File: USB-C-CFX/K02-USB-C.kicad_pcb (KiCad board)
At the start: 2 copper layers, 98.3 x 87.7 mm, 31 parts, among them SW1 SW_Push, SW10 SW_Push, SW11 SW_Push, SW12 SW_Push, SW13 SW_Push, SW14 SW_Push, SW15 SW_Push, SW16 SW_Push, SW17 SW_Push, SW18 SW_Push, SW2 SW_Push, SW3 SW_Push, SW4 SW_Push, SW5 SW_Push, SW6 SW_Push, SW7 SW_Push, SW8 SW_Push, SW9 SW_Push, U1 ProMicro-kbd

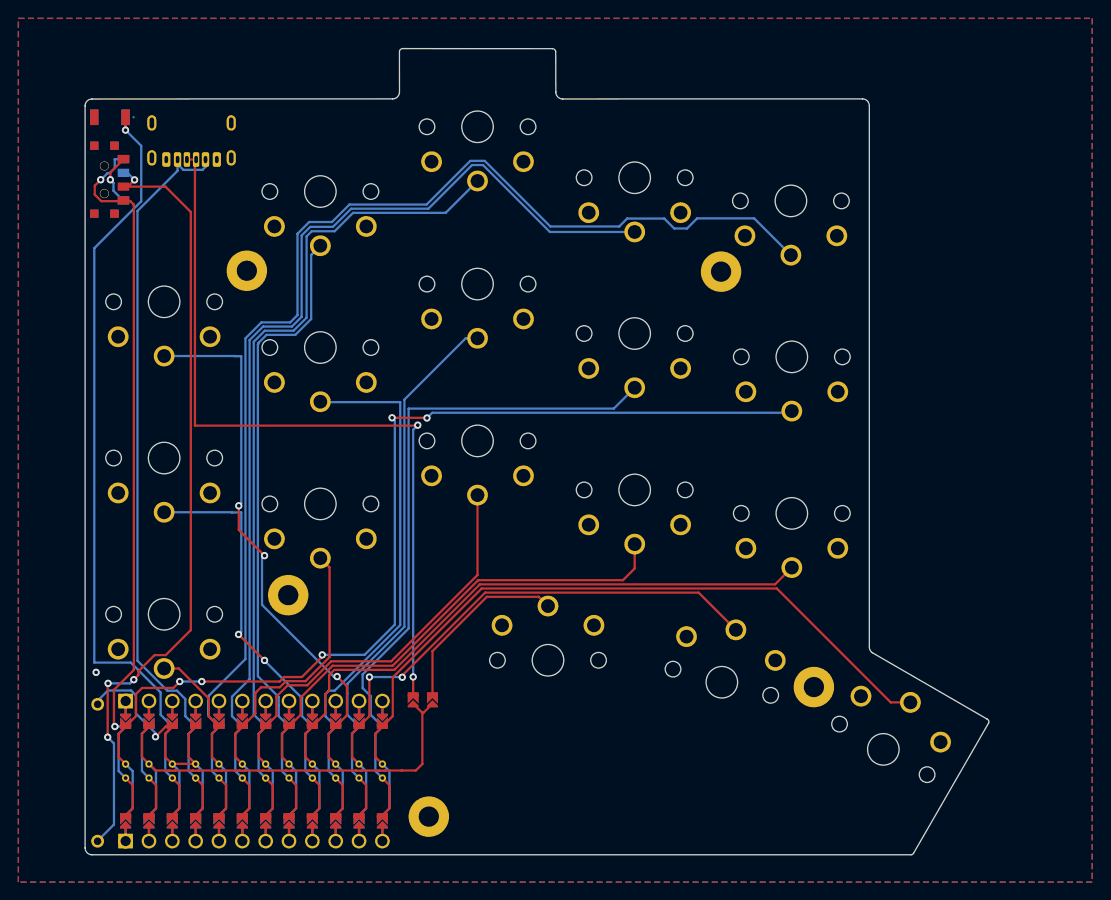
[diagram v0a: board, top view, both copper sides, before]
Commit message: upsie
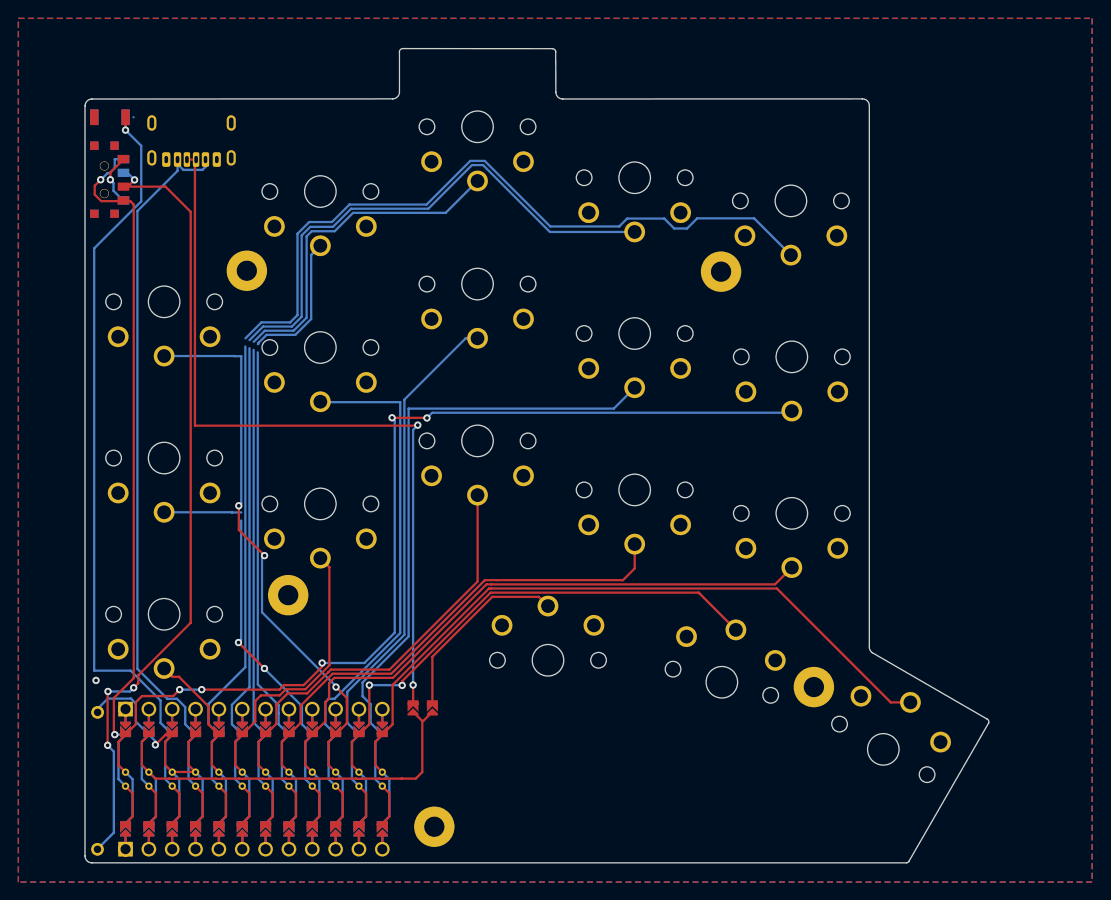
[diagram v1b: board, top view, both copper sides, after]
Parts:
- moved ? 1.25 mm to (60.5, 103.2)
- moved ? 0.88 mm to (58.7, 91.0)
- moved ? 0.88 mm to (60.8, 91.0)
- moved B+ 0.88 mm to (23.9, 105.7)
- moved U1 0.88 mm to (40.9, 98.0)
- moved B- 0.88 mm to (23.9, 90.8)
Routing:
- net Switch10: track 101.9 -> 103.3 mm
- net Switch18: track 143.0 -> 144.4 mm
- net reset: track 76.4 -> 77.2 mm
- net Switch9: track 63.1 -> 64.0 mm
- net Switch8: track 49.4 -> 50.3 mm
- net Switch7: track 48.2 -> 49.1 mm
- net vcc: track 72.5 -> 73.3 mm
- net Switch12: track 25.1 -> 26.0 mm
- net raw: track 69.5 -> 70.3 mm
- net Switch13: track 39.8 -> 40.6 mm
- net Switch16: track 51.3 -> 52.0 mm
- net Switch1: track 54.6 -> 55.3 mm
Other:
- board size 98.3 x 87.7 mm -> 98.4 x 88.6 mm
